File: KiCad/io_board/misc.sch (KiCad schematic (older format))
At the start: 19 parts, among them U6 27C512

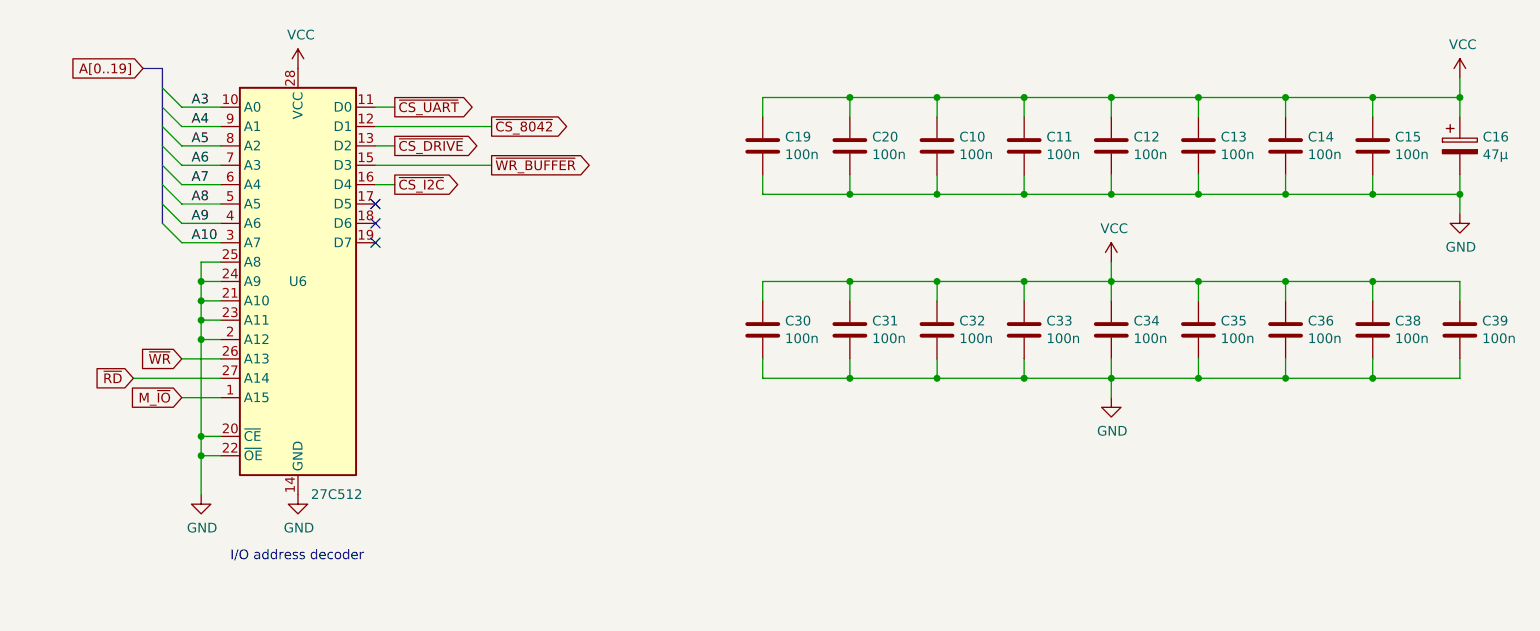
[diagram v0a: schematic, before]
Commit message: Updated I/O board
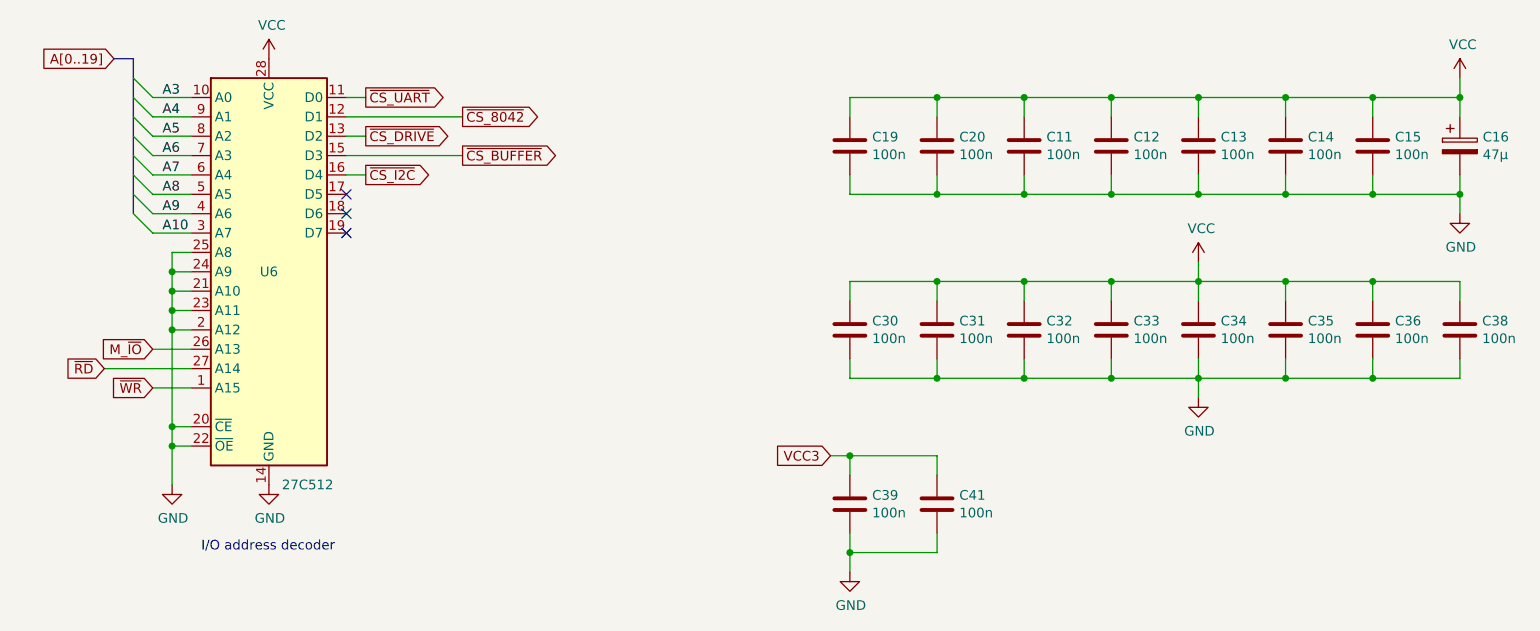
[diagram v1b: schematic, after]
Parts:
- removed C10: 100n, Capacitor_SMD:C_1206_3216Metric, symbol Device:C
- added C41: 100n, Capacitor_SMD:C_1206_3216Metric, symbol Device:C
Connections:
- net GND: now also C41.2
- net M_~IO: now also U6.26 (A13); no longer U6.1 (A15)
- net VCC: no longer C39.1
- net ~WR: now also U6.1 (A15); no longer U6.26 (A13)
- net ~WR_BUFFER renamed ~CS_BUFFER
- new net VCC3: C39.1, C41.1
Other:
- moved on the sheet: C19, C20, C30, C31, C32, C33, C34, C35, C36, C38, C39, U6
